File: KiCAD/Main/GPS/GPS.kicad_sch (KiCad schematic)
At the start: 16 parts, among them U1 MAX-M8Q, U2 PHA-23LN

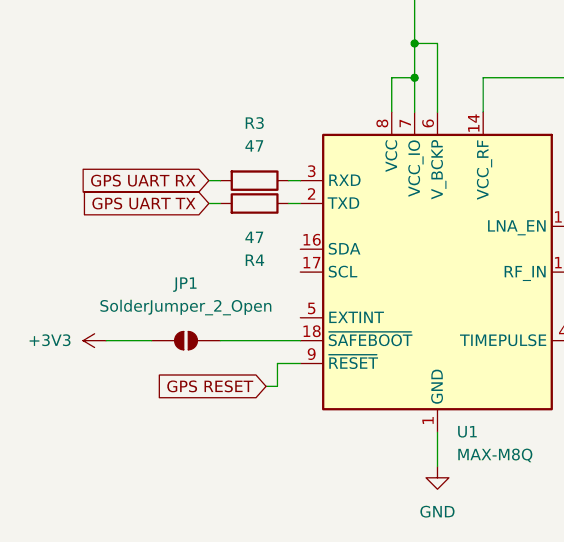
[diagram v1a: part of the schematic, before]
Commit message: Fix labeling issue
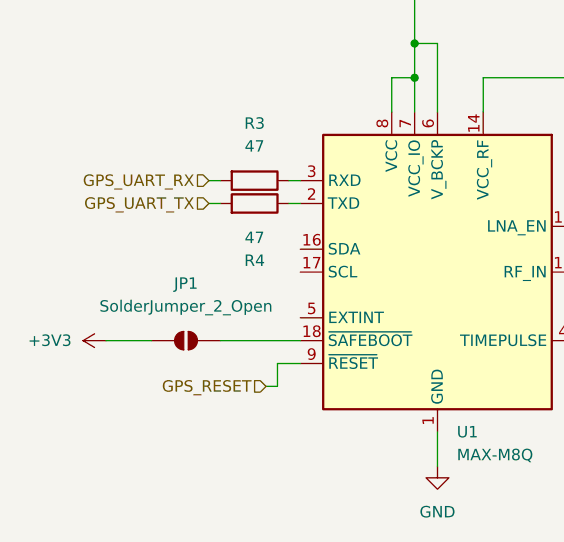
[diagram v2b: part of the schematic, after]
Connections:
- net GPS RESET renamed GPS_RESET
- net GPS UART RX renamed GPS_UART_RX
- net GPS UART TX renamed GPS_UART_TX
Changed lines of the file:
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@@
 		)
 	)
-	(global_label "GPS UART TX"
+	(hierarchical_label "GPS_UART_TX"
 		(shape input)
 		(at 73.66 68.58 180)
-		(fields_autoplaced yes)
 		(effects
 			(font
@@
 			(justify right)
 		)
-		(property "Intersheetrefs" "${INTERSHEET_REFS}"
-			(at 58.1563 68.58 0)
-			(effects
-				(font
-					(size 1.27 1.27)
-				)
-				(justify right)
-				(hide yes)
-			)
-		)
 	)
-	(global_label "GPS UART RX"
+	(hierarchical_label "GPS_RESET"
 		(shape input)
-		(at 73.66 66.04 180)
-		(fields_autoplaced yes)
+		(at 80.01 88.9 180)
 		(effects
 			(font
@@
 			(justify right)
 		)
-		(property "Intersheetrefs" "${INTERSHEET_REFS}"
-			(at 57.8539 66.04 0)
-			(effects
-				(font
-					(size 1.27 1.27)
-				)
-				(justify right)
-				(hide yes)
-			)
-		)
 	)
-	(global_label "GPS RESET"
+	(hierarchical_label "GPS_UART_RX"
 		(shape input)
-		(at 80.01 88.9 180)
-		(fields_autoplaced yes)
+		(at 73.66 66.04 180)
 		(effects
 			(font
@@
 			(justify right)
 		)
-		(property "Intersheetrefs" "${INTERSHEET_REFS}"
-			(at 66.5626 88.9 0)
-			(effects
-				(font
-					(size 1.27 1.27)
-				)
-				(justify right)
-				(hide yes)
-			)
-		)
 	)

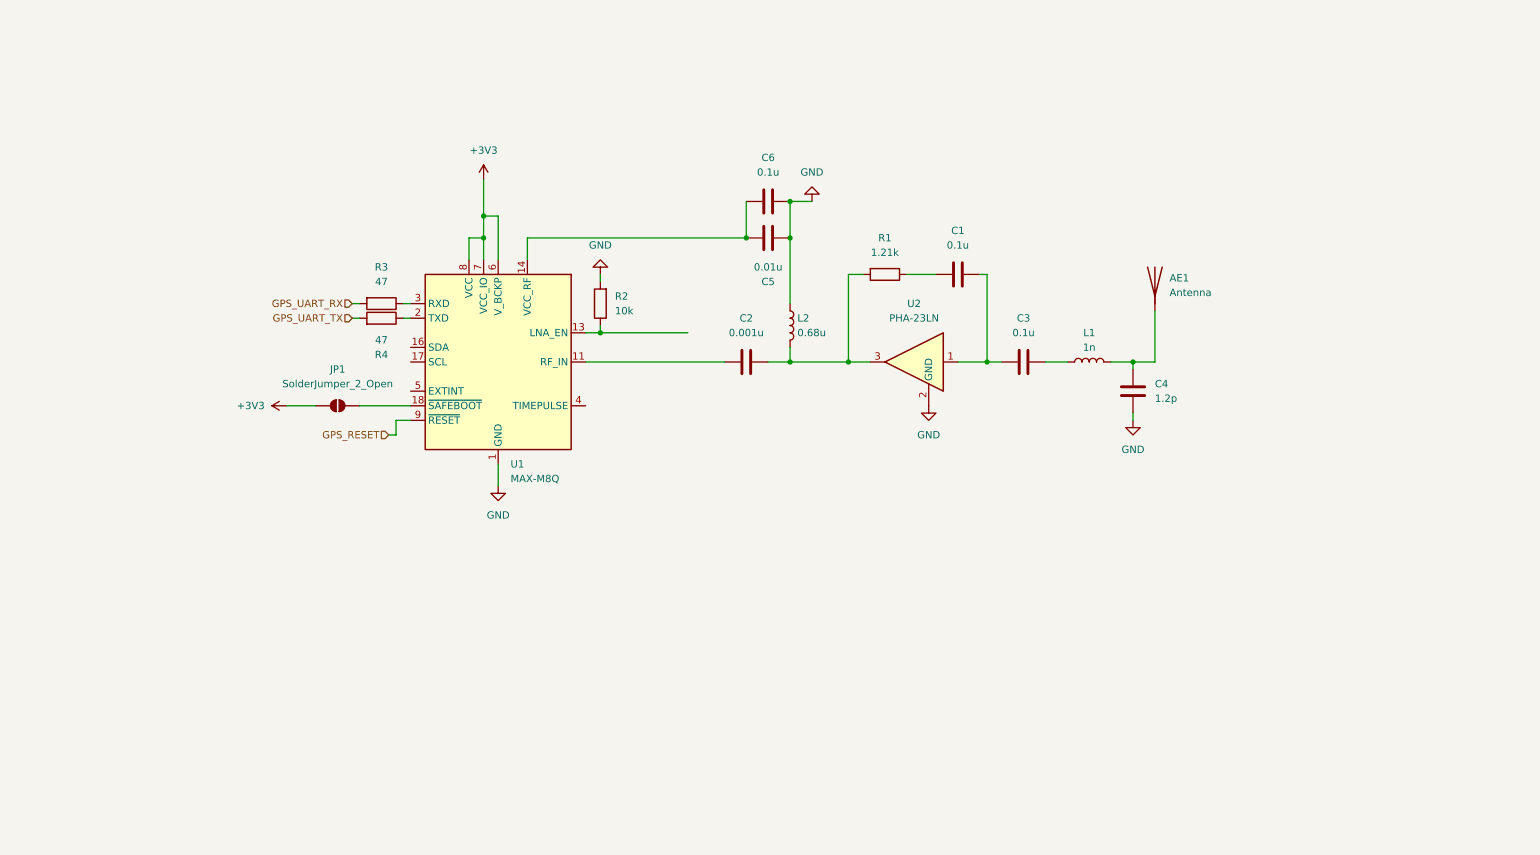
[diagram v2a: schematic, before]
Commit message: Continue integrating
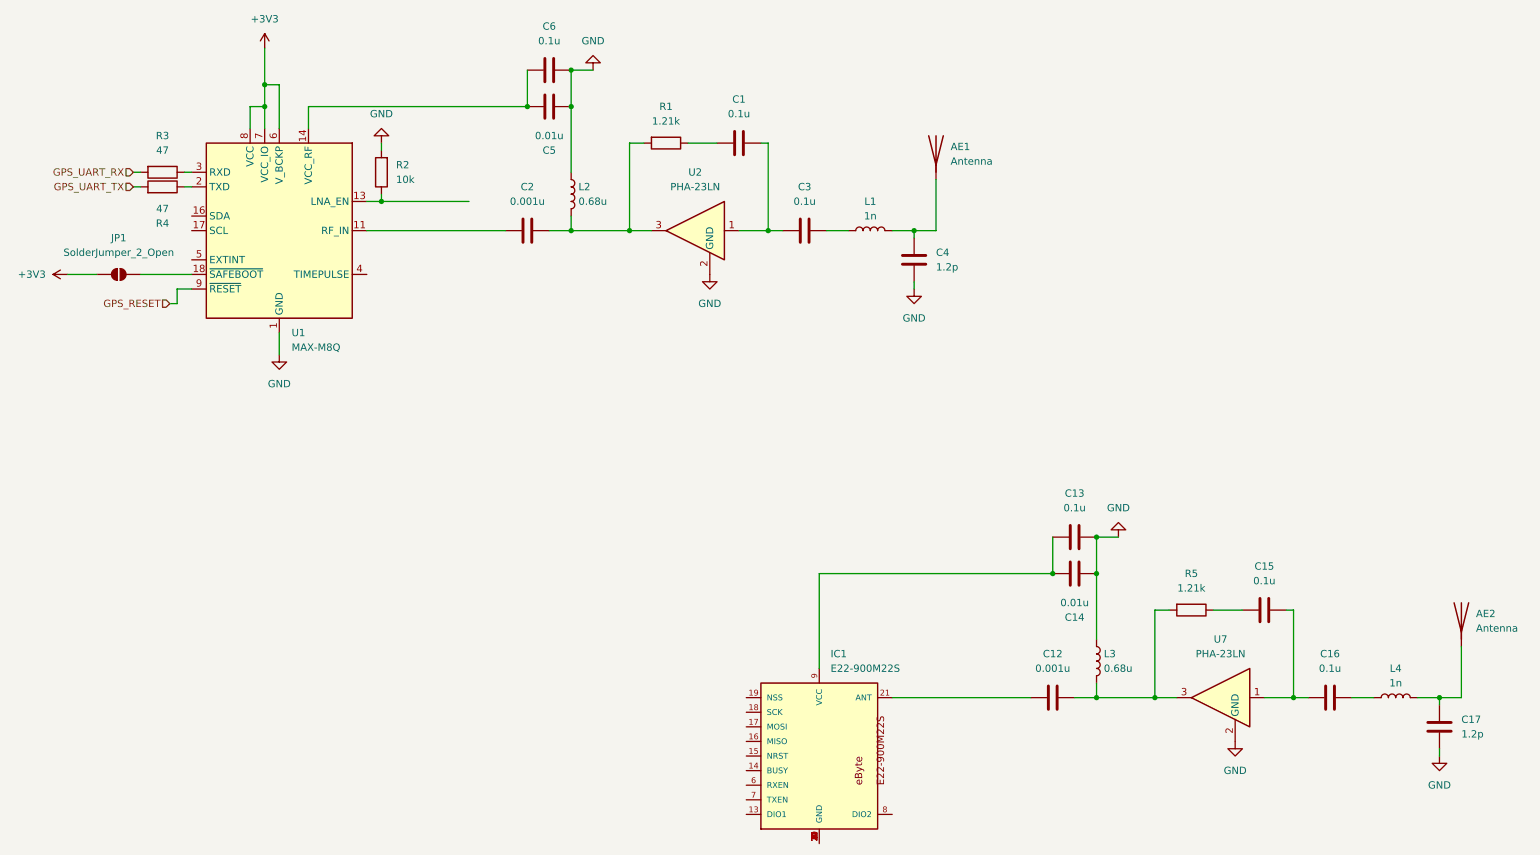
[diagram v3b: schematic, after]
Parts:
- added AE2: Antenna, symbol Device:Antenna
- added C12: 0.001u, symbol Device:C
- added C13, C15, C16: 0.1u, symbol Device:C
- added C14: 0.01u, symbol Device:C
- added C17: 1.2p, symbol Device:C
- added IC1: E22-900M22S, E22-900M22S:E22-900M22S, symbol E22-900M22S:E22-900M22S
- added L3: 0.68u, symbol Device:L
- added L4: 1n, symbol Device:L
- added R5: 1.21k, symbol Device:R
- added U7: PHA-23LN, Package_TO_SOT_SMD:SOT-89-3, symbol RF_Amplifier:PHA-23LN
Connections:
- net GND: now also C13.1, C14.1, C17.2, L3.1, U7.2 (GND)
- new net: C13.2, C14.2, IC1.9 (VCC)
- new net: C15.1, R5.1
- new net: C12.2, L3.2, R5.2, U7.3
- new net: AE2.1 (A), C17.1, L4.2
- new net: C12.1, IC1.21 (ANT)
- new net: C15.2, C16.2, U7.1
- new net: C16.1, L4.1
- new net: IC1.1 (GND), IC1.10 (GND), IC1.11 (GND), IC1.12 (GND), IC1.2 (GND), IC1.20 (GND), IC1.22 (GND), IC1.3 (GND), IC1.4 (GND), IC1.5 (GND)
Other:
- moved on the sheet: AE1, C1, C2, C3, C4, C5, C6, JP1, L1, L2, R1, R2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
